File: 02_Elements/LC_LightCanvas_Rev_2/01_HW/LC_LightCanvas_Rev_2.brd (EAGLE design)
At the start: 132 x 100 mm, 86 parts

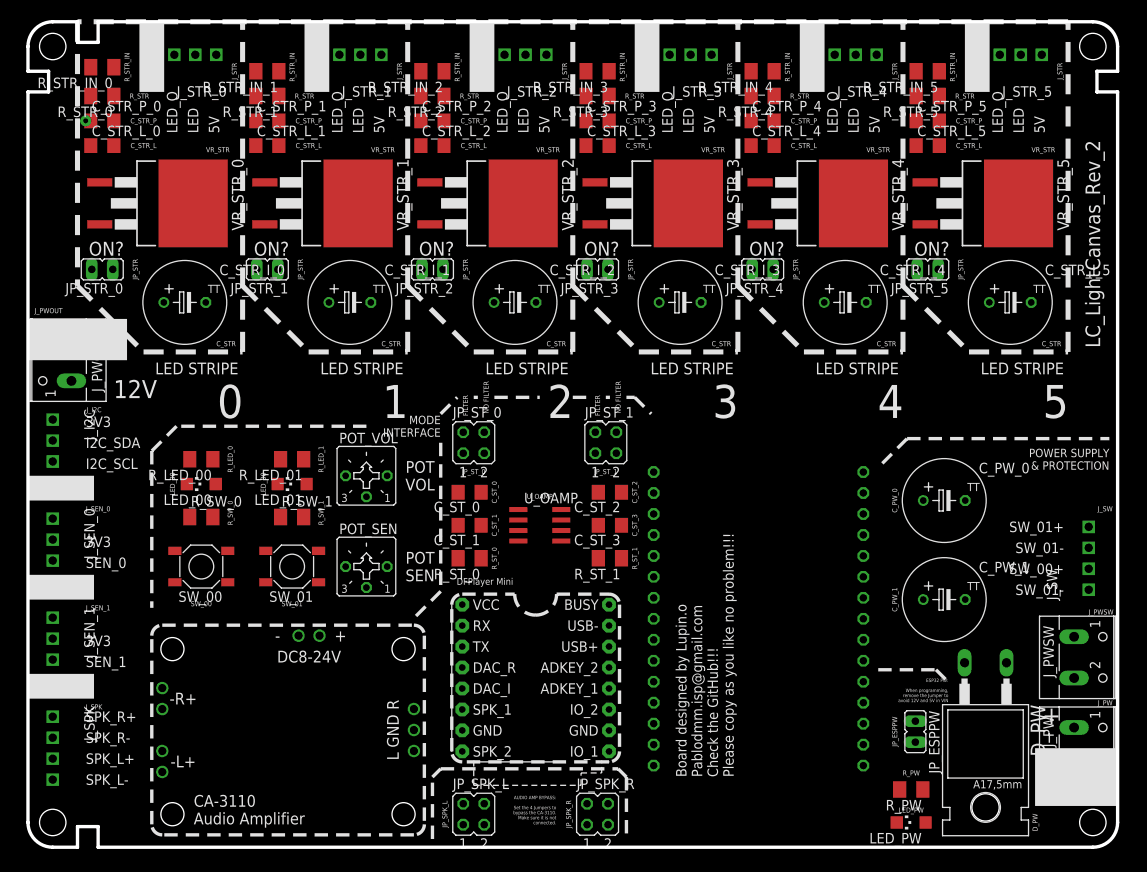
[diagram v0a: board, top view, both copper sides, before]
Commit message: Fix of HW and Gerber Files
Fixed HW
Generation of Gerber Files
Generation of 3D Model
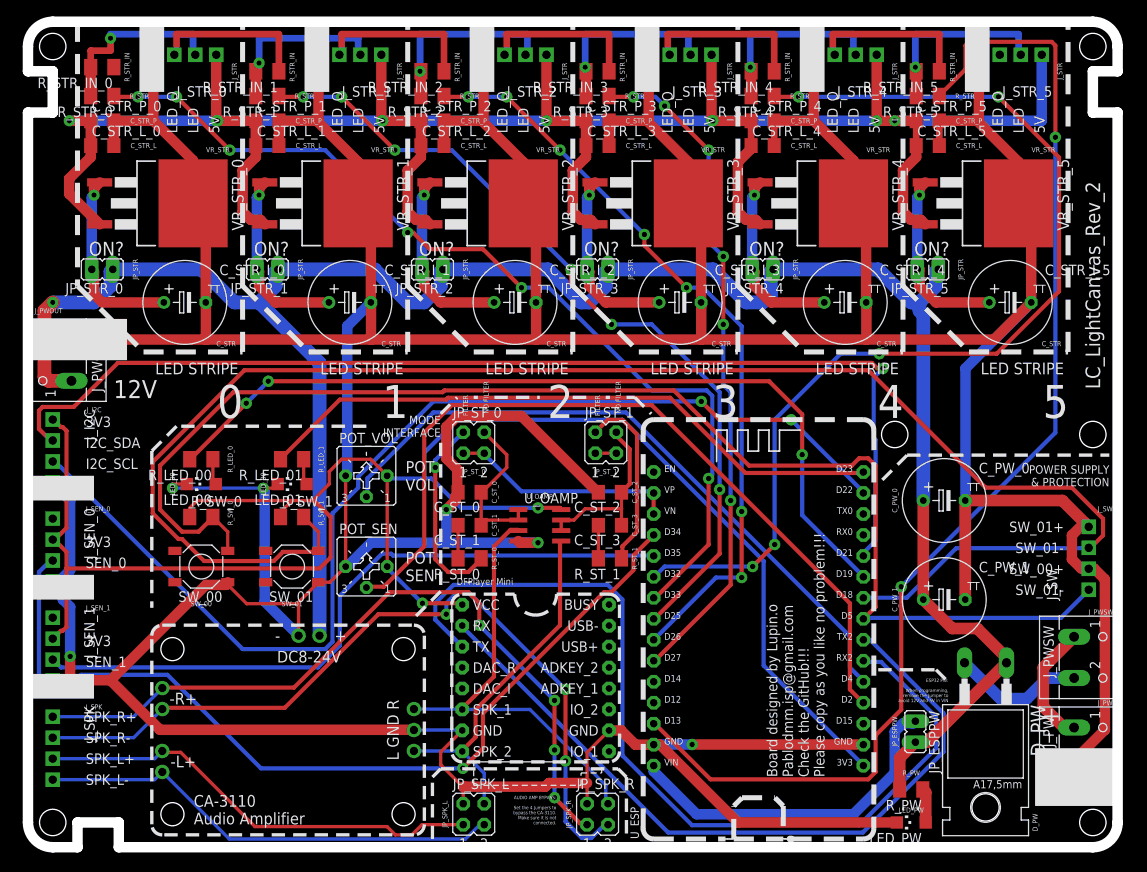
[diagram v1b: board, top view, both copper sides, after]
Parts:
- flipped U_ESP to the top
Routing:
- net GND: track 0.00 -> 832.7 mm, vias 0 -> 6
- net VOUT: track 0.00 -> 280.1 mm, vias 0 -> 10
- net VIN_12V: track 0.00 -> 259.8 mm, vias 0 -> 1
- net 3V3: track 0.00 -> 229.8 mm, vias 0 -> 2
- net SW_01: track 0.00 -> 195.4 mm
- net SW_00: track 0.00 -> 161.3 mm
- net LED_STR_5: track 0.00 -> 145.7 mm, vias 0 -> 2
- net I2C_SCL: track 0.00 -> 134.7 mm, vias 0 -> 2
- net I2C_SDA: track 0.00 -> 133.4 mm, vias 0 -> 1
- net LED_STR_4: track 0.00 -> 126.1 mm, vias 0 -> 5
- net LED_STR_0: track 0.00 -> 115.1 mm, vias 0 -> 6
- net SEN_0: track 0.00 -> 112.3 mm, vias 0 -> 1
- net MP3_TX: track 0.00 -> 110.6 mm
- net LED_00: track 0.00 -> 102.5 mm, vias 0 -> 3
- net LED_STR_1: track 0.00 -> 100.1 mm, vias 0 -> 6
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- added copper zone on layer 1, net GND
- added copper zone on layer 16, net GND
- added copper zone on layer 1, net N$11
- added copper zone on layer 16, net N$28
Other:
- outline, holes or cut-outs redrawn
